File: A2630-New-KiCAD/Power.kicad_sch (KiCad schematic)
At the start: 27 parts, among them U204 74HCT04, U300 74HCT05, U307 74HCT04, U507 74HCT74, U606 74HCT244, U800 LM1117-3.3

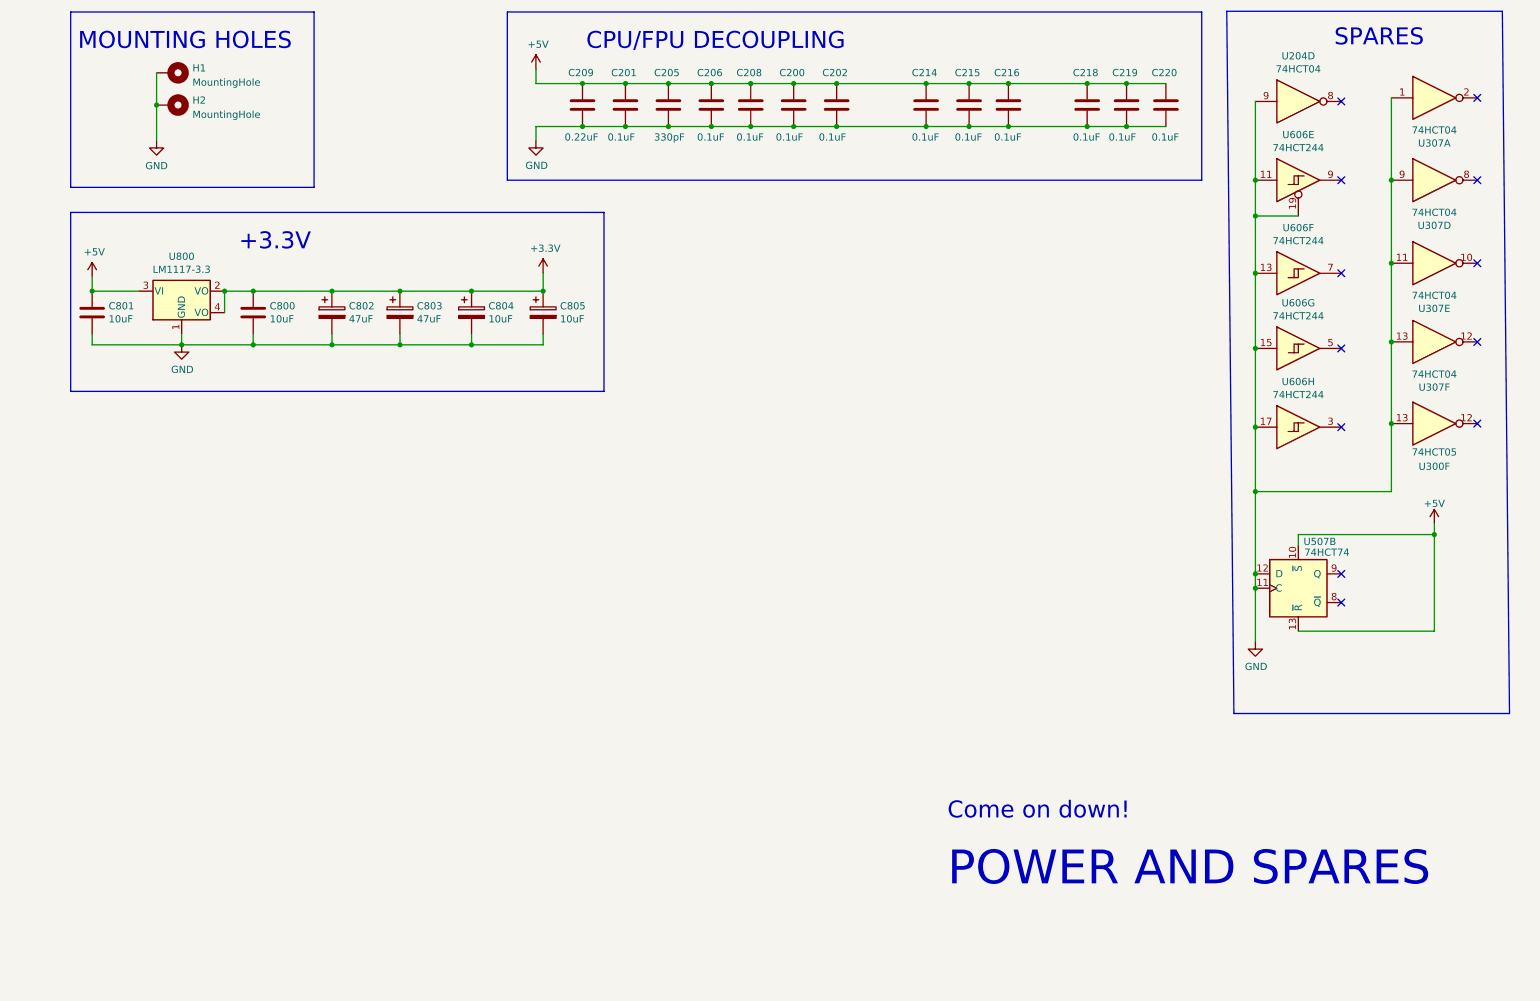
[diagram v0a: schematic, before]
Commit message: Add files via upload
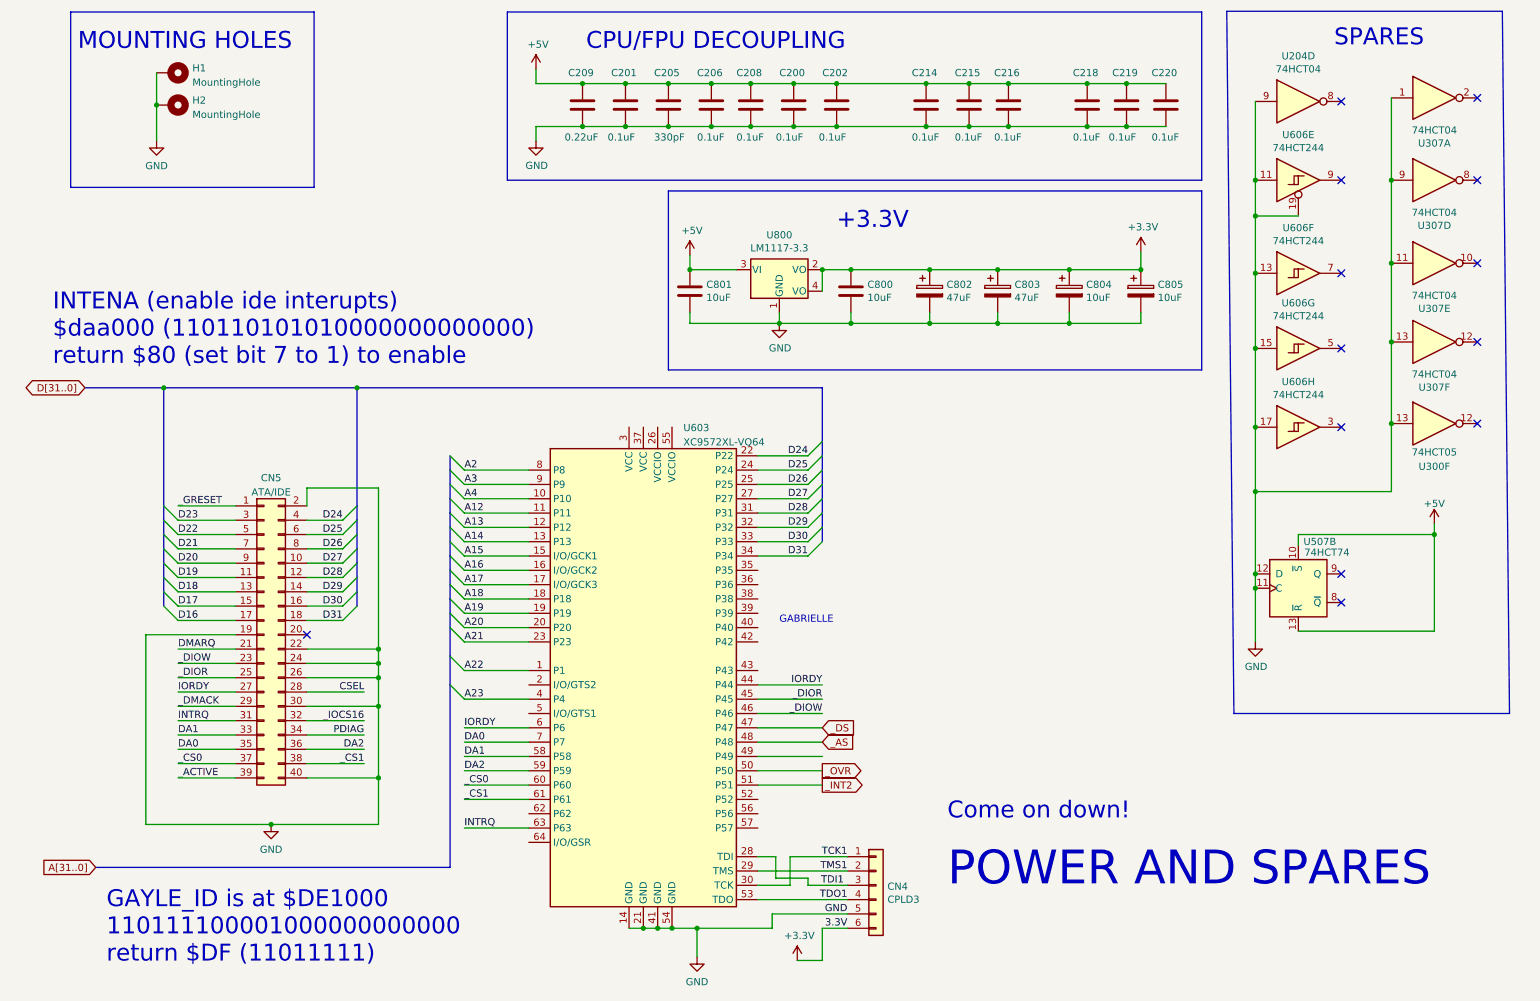
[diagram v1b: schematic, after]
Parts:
- added CN4: CPLD3, Connector_PinHeader_2.54mm:PinHeader_1x06_P2.54mm_Vertical, symbol Connector_Generic:Conn_01x06
- added CN5: ATA/IDE, N2630:ATA_Header_2x20_P2.54mm, symbol Connector_Generic:Conn_02x20_Odd_Even
- added U603: XC9572XL-VQ64, Package_QFP:TQFP-64_10x10mm_P0.5mm, symbol CPLD_Xilinx:XC9572XL-VQ64
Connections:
- net +3V3: now also CN4.6 (Pin_6)
- net GND: now also CN4.5 (Pin_5), CN5.19 (Pin_19), CN5.2 (Pin_2), CN5.22 (Pin_22), CN5.24 (Pin_24), CN5.26 (Pin_26), CN5.30 (Pin_30), CN5.40 (Pin_40), U603.14 (GND), U603.21 (GND), U603.41 (GND), U603.54 (GND)
- new net A12: U603.11 (P11)
- new net A13: U603.12 (P12)
- new net A14: U603.13 (P13)
- new net A15: U603.15 (I/O/GCK1)
- new net A16: U603.16 (I/O/GCK2)
- new net A17: U603.17 (I/O/GCK3)
- new net A18: U603.18 (P18)
- new net A19: U603.19 (P19)
- new net A2: U603.8 (P8)
- new net A20: U603.20 (P20)
- new net A21: U603.23 (P23)
- new net A22: U603.1 (P1)
- new net A23: U603.4 (P4)
- new net A3: U603.9 (P9)
- new net A4: U603.10 (P10)
- new net CSEL: CN5.28 (Pin_28)
- new net D16: CN5.17 (Pin_17)
- new net D17: CN5.15 (Pin_15)
- new net D18: CN5.13 (Pin_13)
- new net D19: CN5.11 (Pin_11)
- new net D20: CN5.9 (Pin_9)
- new net D21: CN5.7 (Pin_7)
- new net D22: CN5.5 (Pin_5)
- new net D23: CN5.3 (Pin_3)
- new net D24: CN5.4 (Pin_4), U603.22 (P22)
- new net D25: CN5.6 (Pin_6), U603.24 (P24)
- new net D26: CN5.8 (Pin_8), U603.25 (P25)
- new net D27: CN5.10 (Pin_10), U603.27 (P27)
- new net D28: CN5.12 (Pin_12), U603.31 (P31)
- new net D29: CN5.14 (Pin_14), U603.32 (P32)
- new net D30: CN5.16 (Pin_16), U603.33 (P33)
- new net D31: CN5.18 (Pin_18), U603.34 (P34)
- new net DA0: CN5.35 (Pin_35), U603.7 (P7)
- new net DA1: CN5.33 (Pin_33), U603.58 (P58)
- new net DA2: CN5.36 (Pin_36), U603.59 (P59)
- new net DMARQ: CN5.21 (Pin_21)
- new net INTRQ: CN5.31 (Pin_31), U603.63 (P63)
- new net IORDY: CN5.27 (Pin_27), U603.44 (P44), U603.6 (P6)
- new net PDIAG: CN5.34 (Pin_34)
- new net TCK1: CN4.1 (Pin_1), U603.30 (TCK)
- new net TDI1: CN4.3 (Pin_3), U603.28 (TDI)
- new net TDO1: CN4.4 (Pin_4), U603.53 (TDO)
- new net TMS1: CN4.2 (Pin_2), U603.29 (TMS)
- new net _ACTIVE: CN5.39 (Pin_39)
- new net _AS: U603.48 (P48)
- new net _CS0: CN5.37 (Pin_37), U603.60 (P60)
- new net _CS1: CN5.38 (Pin_38), U603.61 (P61)
- new net _DIOR: CN5.25 (Pin_25), U603.45 (P45)
- new net _DIOW: CN5.23 (Pin_23), U603.46 (P46)
- new net _DMACK: CN5.29 (Pin_29)
- new net _DS: U603.47 (P47)
- new net _GRESET: CN5.1 (Pin_1)
- new net _INT2: U603.51 (P51)
- new net _IOCS16: CN5.32 (Pin_32)
- new net _OVR: U603.50 (P50)
- no-connect marks 12 -> 13
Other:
- note added: "GABRIELLE"
- note added: "GAYLE_ID is at $DE1000 110111100001000000000000 return $DF (11011111)"
- note added: "INTENA (enable ide interupts) $daa000 (110110101010000000000000) return $80 (set bit 7 to 1) to enable"
- moved on the sheet: C800, C801, C802, C803, C804, C805, U800
